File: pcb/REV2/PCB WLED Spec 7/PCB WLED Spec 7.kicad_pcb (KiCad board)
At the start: 2 copper layers, 12 parts, among them J1 USB_C_Receptacle_USB2.0_16P, U1 ESP32-C3, U2 RT9013-33GB, U3 LMR14050SDDAR

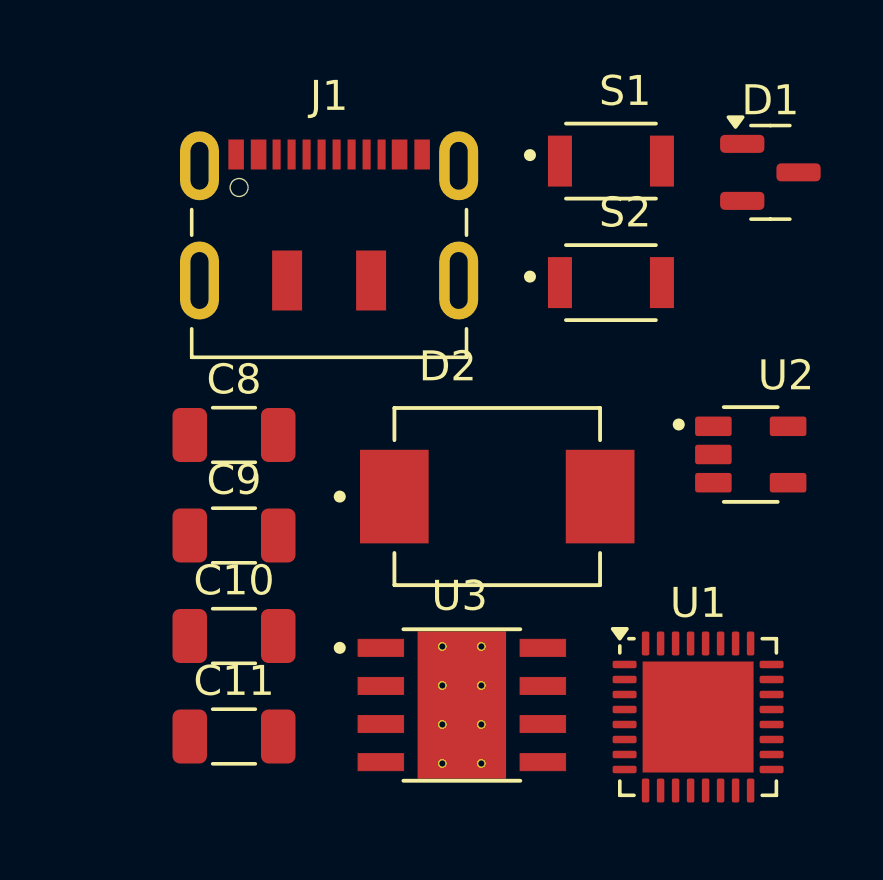
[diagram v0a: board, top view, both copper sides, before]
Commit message: Update PCB WLED Spec 7.kicad_pcb
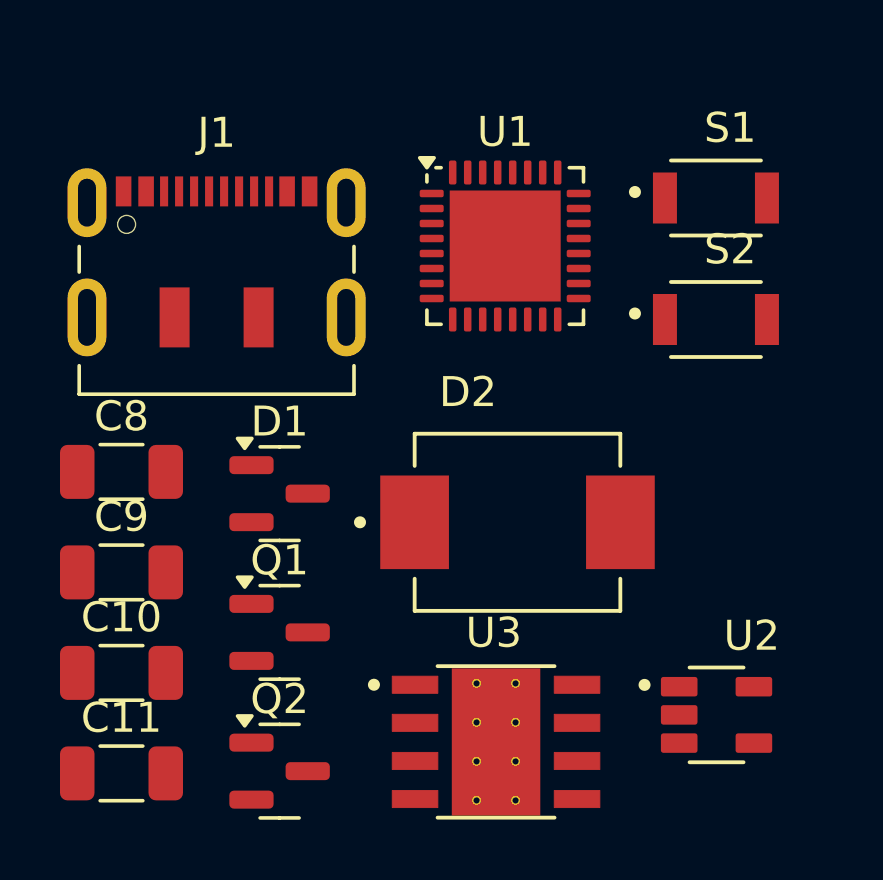
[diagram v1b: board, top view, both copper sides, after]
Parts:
- added Q1: BC807, Package_TO_SOT_SMD:SOT-23, F.Cu at (163.1, 134.8)
- added Q2: BC807, Package_TO_SOT_SMD:SOT-23, F.Cu at (163.1, 139.5)
- moved D1 19.6 mm to (163.1, 130.2)
- moved U1 17.0 mm to (170.6, 122.0)
- moved U2 8.75 mm to (177.6, 137.6)
- moved C10 3.95 mm to (157.8, 136.2)
- moved C9 3.95 mm to (157.8, 132.8)
- moved J1 3.95 mm to (160.9, 123.2)
- moved C11 3.95 mm to (157.8, 139.5)
- moved C8 3.95 mm to (157.8, 129.5)
- moved S2 3.71 mm to (177.6, 124.4)
- moved S1 3.71 mm to (177.6, 120.3)
- moved U3 1.68 mm to (170.3, 138.5)
- moved D2 1.09 mm to (171.0, 131.2)
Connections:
- net Net-(U1-GPIO2) renamed LED1_IN
- U1 pad 16: unconnected-(U1-GPIO10-Pad16) -> LED2_IN
